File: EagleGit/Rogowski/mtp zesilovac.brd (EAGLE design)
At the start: 160 x 100 mm, 25 parts, among them IC1 TL061P, IC2 TL061P, IC3 TL061P, X1 SMKDSP_1,5/2, X2 SMKDSP_1,5/2, X3 SMKDSP_1,5/2, X4 SMKDSP_1,5/2, X5 SMKDSP_1,5/2, X6 SMKDSP_1,5/2, X7 SMKDSP_1,5/2

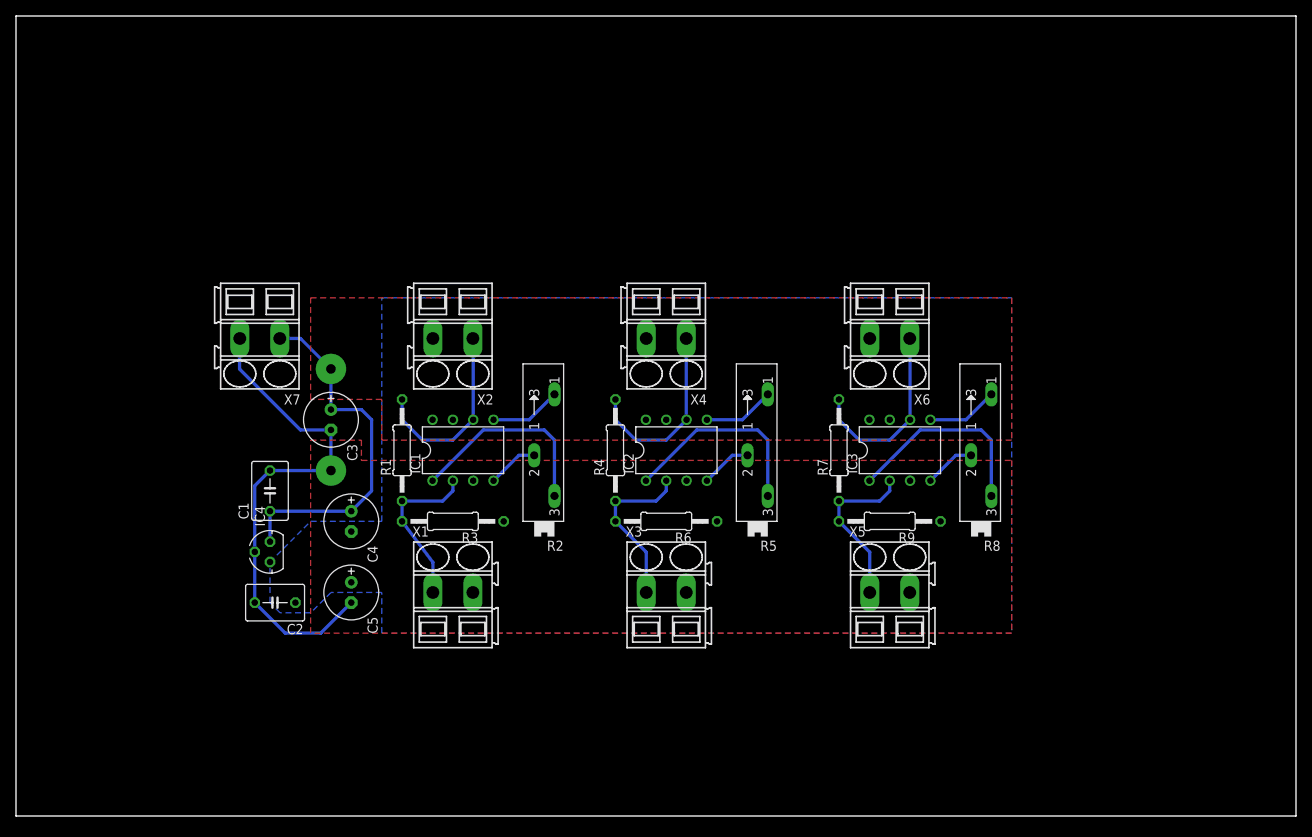
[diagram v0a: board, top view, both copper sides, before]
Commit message: DPS pro akvarko
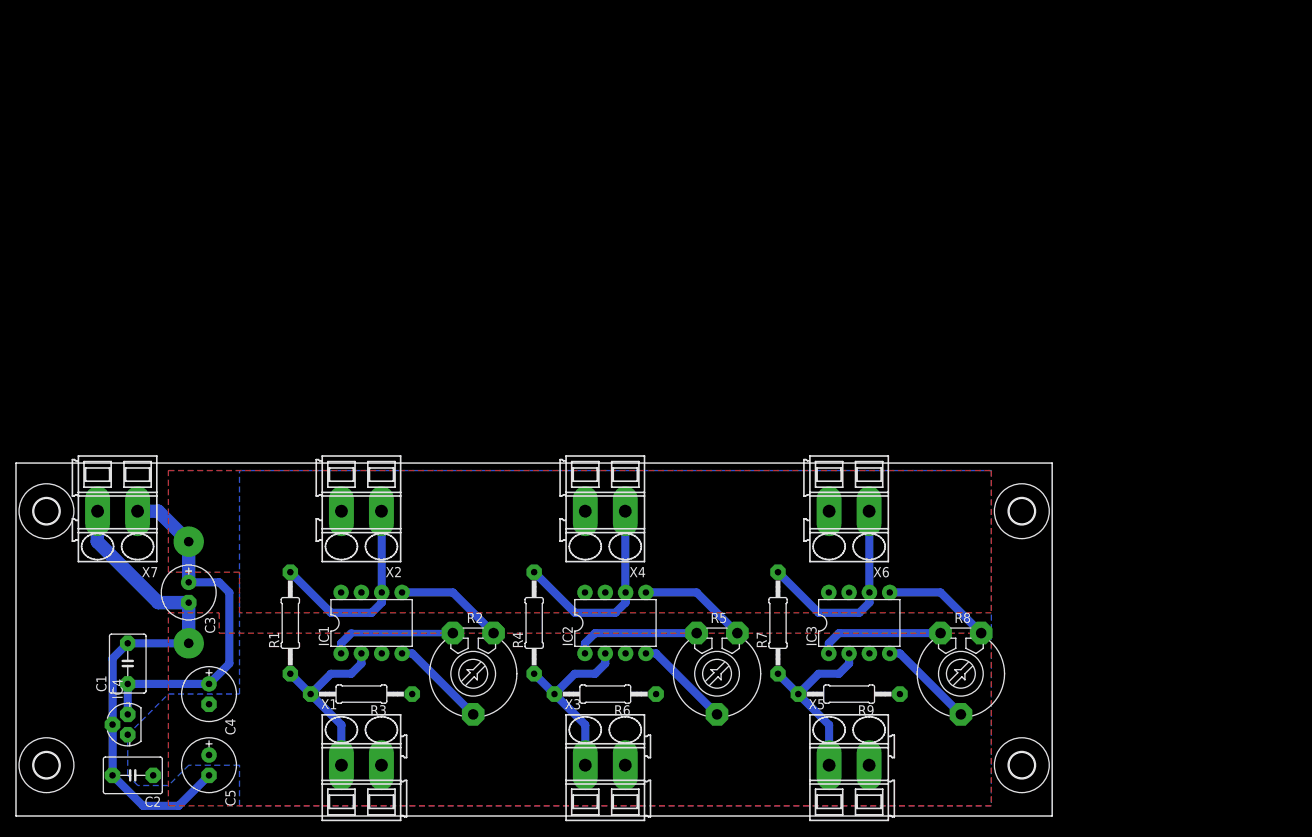
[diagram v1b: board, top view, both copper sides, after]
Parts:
- added U$1, U$2, U$3, U$4: (no value), holes:3,2
- R2, R5, R8: device pot:SP19L -> pot:LI10
- moved R2 30.5 mm to (57.1, 17.8), turned to 180 degrees
- moved R5 29.6 mm to (87.6, 17.8), turned to 180 degrees
- moved R8 29.3 mm to (118.1, 17.8), turned to 180 degrees
- moved IC4 28.0 mm to (14.0, 11.4)
- moved C1 28.0 mm to (14.0, 19.1)
- moved C2 28.0 mm to (14.6, 5.08)
- moved C5 28.0 mm to (24.1, 6.35)
- moved C3 28.0 mm to (21.6, 27.9)
- moved C4 28.0 mm to (24.1, 15.2)
- moved X7 28.0 mm to (12.7, 38.1)
- moved R1 25.7 mm to (34.3, 24.1)
- moved X1 24.4 mm to (43.2, 6.35)
- moved IC1 24.4 mm to (44.5, 24.1)
- moved R3 24.4 mm to (43.2, 15.2)
- moved X2 24.4 mm to (43.2, 38.1)
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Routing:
- net GND: track 82.8 -> 99.8 mm
- net N$12: track 25.4 -> 15.8 mm
- net N$8: track 25.4 -> 15.8 mm
- net N$4: track 25.4 -> 15.8 mm
- net N$7: track 8.94 -> 13.5 mm
- net N$11: track 8.94 -> 13.5 mm
- net N$3: track 8.94 -> 13.5 mm
- net N$1: track 20.9 -> 23.3 mm
- net N$9: track 21.2 -> 23.3 mm
- net N$5: track 21.2 -> 23.3 mm
- net N$6: track 23.7 -> 25.5 mm
- net N$2: track 23.7 -> 25.5 mm
- net N$10: track 26.2 -> 28.0 mm
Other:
- board size 160 x 100 mm -> 129.5 x 44.1 mm
